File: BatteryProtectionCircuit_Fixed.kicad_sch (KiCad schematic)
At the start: 40 parts, among them J2 Conn_01x07_Pin, Q1 NMOS, U2 LM358, U3 LM358, U4 LM321, U6 LMC555xN

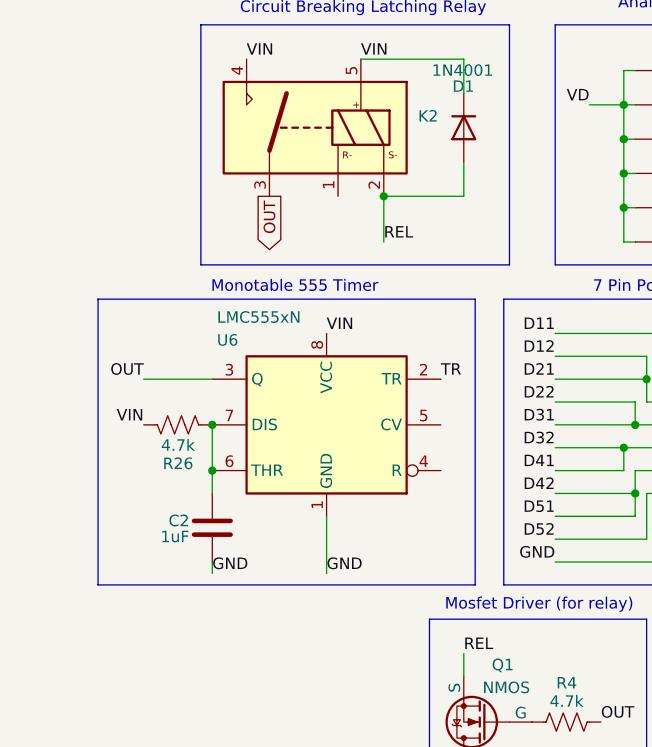
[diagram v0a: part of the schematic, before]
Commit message: Fixed based on Design Review Feedback
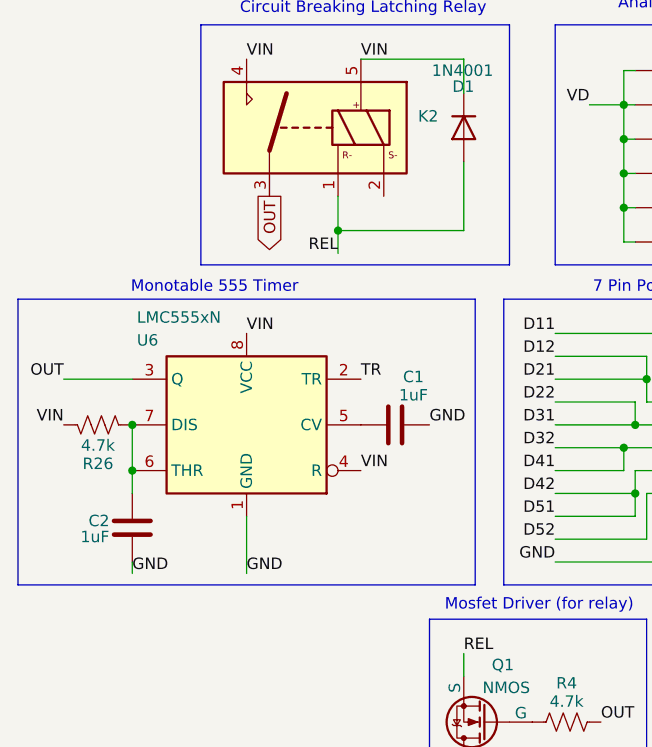
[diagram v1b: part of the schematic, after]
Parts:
- added C1: 1uF, symbol Device:C
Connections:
- net GND: now also C1.2
- net REL: now also K2.1; no longer K2.2
- net VIN: now also U6.4 (R)
- net at U6.5 (CV): now also C1.1
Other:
- moved on the sheet: C2, R26, U6
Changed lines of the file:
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@@
 	)
 	(rectangle
-		(start 85.09 82.55)
+		(start 76.2 82.55)
 		(end 127 114.3)
 		(stroke
@@
 	(text "Monotable 555 Timer"
 		(exclude_from_sim no)
-		(at 106.934 81.28 0)
+		(at 98.044 81.28 0)
 		(effects
 			(font
@@
 	)
 	(junction
+		(at 111.76 74.93)
+		(diameter 0)
+		(color 0 0 0 0)
+	)
+	(junction
 		(at 203.2 104.14)
 		(diameter 0)
@@
 	)
 	(junction
-		(at 97.79 101.6)
+		(at 88.9 101.6)
 		(diameter 0)
 		(color 0 0 0 0)
@@
 	)
 	(junction
-		(at 97.79 96.52)
+		(at 88.9 96.52)
 		(diameter 0)
 		(color 0 0 0 0)
@@
 	)
 	(junction
-		(at 116.84 71.12)
-		(diameter 0)
-		(color 0 0 0 0)
-	)
-	(junction
 		(at 157.48 129.54)
 		(diameter 0)
@@
 	(wire
 		(pts
+			(xy 111.76 74.93) (xy 111.76 71.12)
+		)
+		(stroke
+			(width 0)
+			(type default)
+		)
+	)
+	(wire
+		(pts
 			(xy 191.77 80.01) (xy 187.96 80.01)
 		)
@@
 	(wire
 		(pts
-			(xy 97.79 104.14) (xy 97.79 101.6)
+			(xy 88.9 104.14) (xy 88.9 101.6)
 		)
 		(stroke
@@
 	(wire
 		(pts
+			(xy 111.76 74.93) (xy 111.76 77.47)
+		)
+		(stroke
+			(width 0)
+			(type default)
+		)
+	)
+	(wire
+		(pts
 			(xy 185.42 116.84) (xy 187.96 116.84)
 		)
@@
 	(wire
 		(pts
-			(xy 97.79 101.6) (xy 97.79 96.52)
+			(xy 88.9 101.6) (xy 88.9 96.52)
 		)
 		(stroke
@@
 	(wire
 		(pts
+			(xy 125.73 74.93) (xy 111.76 74.93)
+		)
+		(stroke
+			(width 0)
+			(type default)
+		)
+	)
+	(wire
+		(pts
 			(xy 152.4 68.58) (xy 165.1 68.58)
 		)
@@
 	(wire
 		(pts
-			(xy 116.84 71.12) (xy 116.84 76.2)
-		)
-		(stroke
-			(width 0)
-			(type default)
-		)
-	)
-	(wire
-		(pts
 			(xy 135.89 91.44) (xy 146.05 91.44)
 		)
@@
 	(wire
 		(pts
-			(xy 110.49 106.68) (xy 110.49 113.03)
+			(xy 101.6 106.68) (xy 101.6 113.03)
 		)
 		(stroke
@@
 	(wire
 		(pts
-			(xy 116.84 71.12) (xy 125.73 71.12)
-		)
-		(stroke
-			(width 0)
-			(type default)
-		)
-	)
-	(wire
-		(pts
-			(xy 125.73 71.12) (xy 125.73 67.31)
+			(xy 125.73 67.31) (xy 125.73 74.93)
 		)
 		(stroke
@@
 	(wire
 		(pts
-			(xy 97.79 111.76) (xy 97.79 113.03)
+			(xy 88.9 111.76) (xy 88.9 113.03)
 		)
 		(stroke
@@
 	(wire
 		(pts
-			(xy 90.17 91.44) (xy 97.79 91.44)
+			(xy 81.28 91.44) (xy 88.9 91.44)
 		)
 		(stroke
@@
 	)
 	(label "TR"
-		(at 123.19 91.44 0)
+		(at 114.3 91.44 0)
 		(effects
 			(font
@@
 	)
 	(label "OUT"
-		(at 90.17 91.44 180)
+		(at 81.28 91.44 180)
 		(effects
 			(font
@@
 		)
 	)
+	(label "VIN"
+		(at 114.3 101.6 0)
+		(effects
+			(font
+				(size 1.27 1.27)
+			)
+			(justify left bottom)
+		)
+	)
 	(label "D51"
 		(at 217.17 128.27 0)
@@
 	)
 	(label "VIN"
-		(at 90.17 96.52 180)
+		(at 81.28 96.52 180)
 		(effects
 			(font
@@
 	)
 	(label "VIN"
-		(at 110.49 86.36 0)
+		(at 101.6 86.36 0)
 		(effects
 			(font
@@
 	)
 	(label "GND"
-		(at 97.79 113.03 0)
+		(at 88.9 113.03 0)
 		(effects
 			(font
@@
 	)
 	(label "GND"
-		(at 110.49 113.03 0)
+		(at 101.6 113.03 0)
 		(effects
 			(font
@@
 		)
 	)
+	(label "GND"
+		(at 121.92 96.52 0)
+		(effects
+			(font
+				(size 1.27 1.27)
+			)
+			(justify left bottom)
+		)
+	)
 	(label "VD"
 		(at 166.37 129.54 0)
@@
 	)
 	(label "REL"
-		(at 116.84 76.2 0)
+		(at 111.76 77.47 180)
 		(effects
 			(font
 				(size 1.27 1.27)
 			)
-			(justify left bottom)
+			(justify right bottom)
 		)
 	)
@@
 	)
 	(symbol
+		(lib_id "Device:C")
+		(at 118.11 96.52 90)
+		(unit 1)
+		(exclude_from_sim no)
+		(in_bom yes)
+		(on_board yes)
+		(dnp no)
+		(property "Reference" "C1"
+			(at 120.142 91.186 90)
+			(effects
+				(font
+					(size 1.27 1.27)
+				)
+			)
+		)
+		(property "Value" "1uF"
+			(at 120.142 93.218 90)
+			(effects
+				(font
+					(size 1.27 1.27)
+				)
+			)
+		)
+		(property "Footprint" ""
+			(at 121.92 95.5548 0)
+			(effects
+				(font
+					(size 1.27 1.27)
+				)
+				(hide yes)
+			)
+		)
+		(property "Datasheet" "~"
+			(at 118.11 96.52 0)
+			(effects
+				(font
+					(size 1.27 1.27)
+				)
+				(hide yes)
+			)
+		)
+		(property "Description" "Unpolarized capacitor"
+			(at 118.11 96.52 0)
+			(effects
+				(font
+					(size 1.27 1.27)
+				)
+				(hide yes)
+			)
+		)
+		(pin "2"
+		)
+		(pin "1"
+		)
+		(instances
+			(project ""
+				(path "/299dddd9-ac06-42a6-950e-710b9bcf8f9e"
+					(reference "C1")
+					(unit 1)
+				)
+			)
+		)
+	)
+	(symbol
 		(lib_id "Device:R_US")
 		(at 165.1 124.46 0)
@@
 	(symbol
 		(lib_id "Device:C")
-		(at 97.79 107.95 0)
+		(at 88.9 107.95 0)
 		(mirror x)
 		(unit 1)
@@
 		(dnp no)
 		(property "Reference" "C2"
-			(at 95.25 107.188 0)
+			(at 86.36 107.188 0)
 			(effects
 				(font
@@
 		)
 		(property "Value" "1uF"
-			(at 95.25 108.966 0)
+			(at 86.36 108.966 0)
 			(effects
 				(font
@@
 		)
 		(property "Footprint" "Capacitor_SMD:C_0805_2012Metric"
-			(at 98.7552 104.14 0)
+			(at 89.8652 104.14 0)
 			(effects
 				(font
@@
 		)
 		(property "Datasheet" "~"
-			(at 97.79 107.95 0)
+			(at 88.9 107.95 0)
 			(effects
 				(font
@@
 		)
 		(property "Description" "Unpolarized capacitor"
-			(at 97.79 107.95 0)
+			(at 88.9 107.95 0)
 			(effects
 				(font
@@
 	(symbol
 		(lib_id "Timer:LMC555xN")
-		(at 110.49 96.52 0)
+		(at 101.6 96.52 0)
 		(mirror y)
 		(unit 1)
@@
 		(dnp no)
 		(property "Reference" "U6"
-			(at 98.298 87.122 0)
+			(at 89.408 87.122 0)
 			(effects
 				(font
@@
 		)
 		(property "Value" "LMC555xN"
-			(at 98.298 84.582 0)
+			(at 89.408 84.582 0)
 			(effects
 				(font
@@
 		)
 		(property "Footprint" "Package_DIP:DIP-8_W7.62mm"
-			(at 93.98 106.68 0)
+			(at 85.09 106.68 0)
 			(effects
 				(font
@@
 		)
 		(property "Datasheet" "http://www.ti.com/lit/ds/symlink/lmc555.pdf"
-			(at 88.9 106.68 0)
+			(at 80.01 106.68 0)
 			(effects
 				(font
@@
 		)
 		(property "Description" "CMOS Timer, 555 compatible, PDIP-8"
-			(at 110.49 96.52 0)
+			(at 101.6 96.52 0)
 			(effects
 				(font
@@
 	(symbol
 		(lib_id "Device:R_US")
-		(at 93.98 96.52 90)
+		(at 85.09 96.52 90)
 		(mirror x)
 		(unit 1)
@@
 		(dnp no)
 		(property "Reference" "R26"
-			(at 93.98 100.838 90)
+			(at 85.09 100.838 90)
 			(effects
 				(font
@@
 		)
 		(property "Value" "4.7k"
-			(at 93.98 98.806 90)
+			(at 85.09 98.806 90)
 			(effects
 				(font
@@
 		)
 		(property "Footprint" "Resistor_SMD:R_0805_2012Metric"
-			(at 94.234 97.536 90)
+			(at 85.344 97.536 90)
 			(effects
 				(font
@@
 		)
 		(property "Datasheet" "~"
-			(at 93.98 96.52 0)
+			(at 85.09 96.52 0)
 			(effects
 				(font
@@
 		)
 		(property "Description" "Resistor, US symbol"
-			(at 93.98 96.52 0)
+			(at 85.09 96.52 0)
 			(effects
 				(font
